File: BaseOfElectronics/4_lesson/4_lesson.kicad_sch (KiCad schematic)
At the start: 5 parts, among them Q1 BC327, SW1 SW_Push

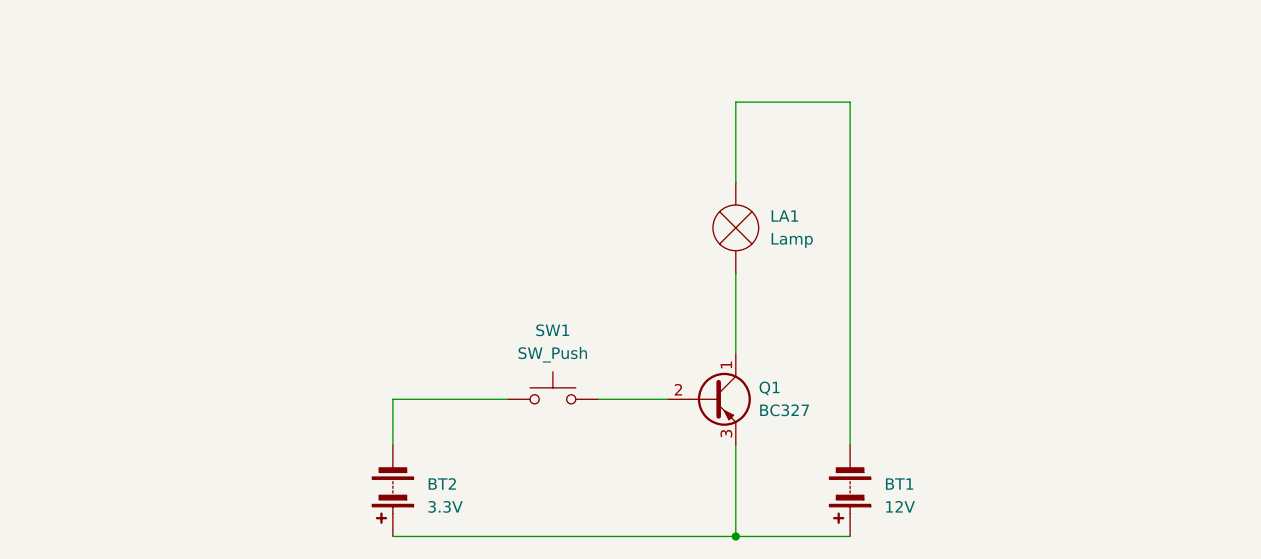
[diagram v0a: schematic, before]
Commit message: add new
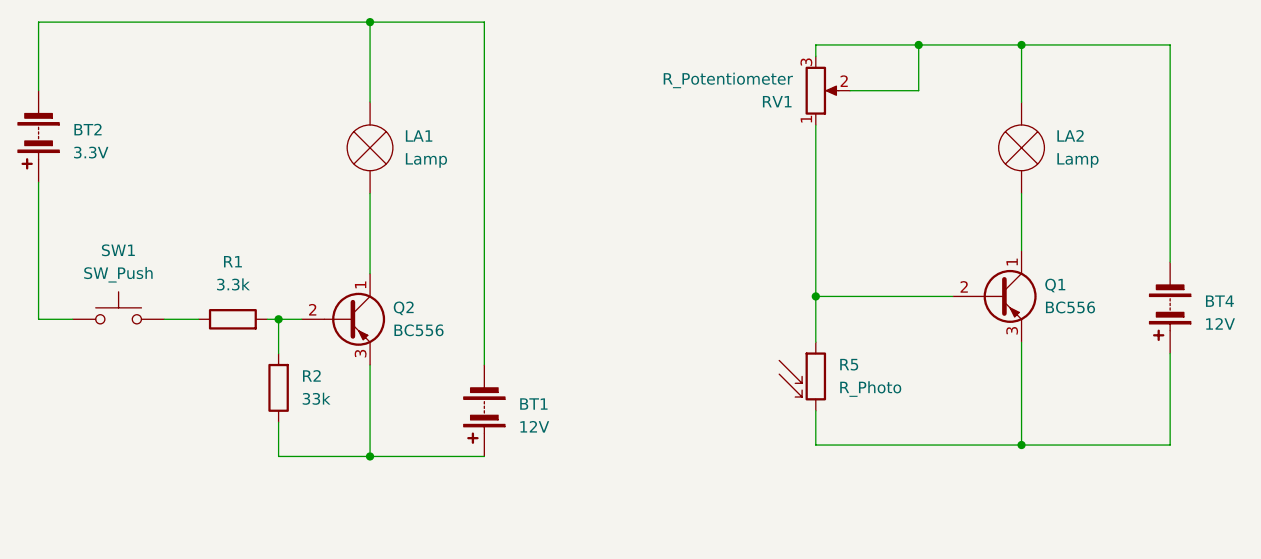
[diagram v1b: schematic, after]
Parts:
- removed Q1: BC327, Package_TO_SOT_THT:TO-92_Inline, symbol Transistor_BJT:BC327
- added BT4: 12V, symbol Device:Battery
- added LA2: Lamp, symbol Device:Lamp
- added Q1, Q2: BC556, Package_TO_SOT_THT:TO-92_Inline, symbol Transistor_BJT:BC556
- added R1: 3.3k, symbol Device:R
- added R2: 33k, symbol Device:R
- added R5: R_Photo, symbol Device:R_Photo
- added RV1: R_Potentiometer, symbol Device:R_Potentiometer
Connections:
- net at LA1.1 (-): now also Q2.1 (C)
- net at SW1.2: now also R1.1
- net at BT1.1 (+): now also Q2.3 (E), R2.1; no longer BT2.1 (+)
- net at BT1.2 (-), LA1.2 (+): now also BT2.2 (-)
- net at SW1.1: now also BT2.1 (+); no longer BT2.2 (-)
- new net: Q1.2 (B), R5.1, RV1.1
- new net: BT4.1 (+), Q1.3 (E), R5.2
- new net: LA2.1 (-), Q1.1 (C)
- new net: BT4.2 (-), LA2.2 (+), RV1.2, RV1.3
- new net: Q2.2 (B), R1.2, R2.2
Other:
- moved on the sheet: BT1, BT2, LA1, SW1
